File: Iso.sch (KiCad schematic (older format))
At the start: 16 parts, among them U11 SN74LVC2G14DBV, U12 4N35S, U13 4N35S, U14 SN74LVC2G14DBV

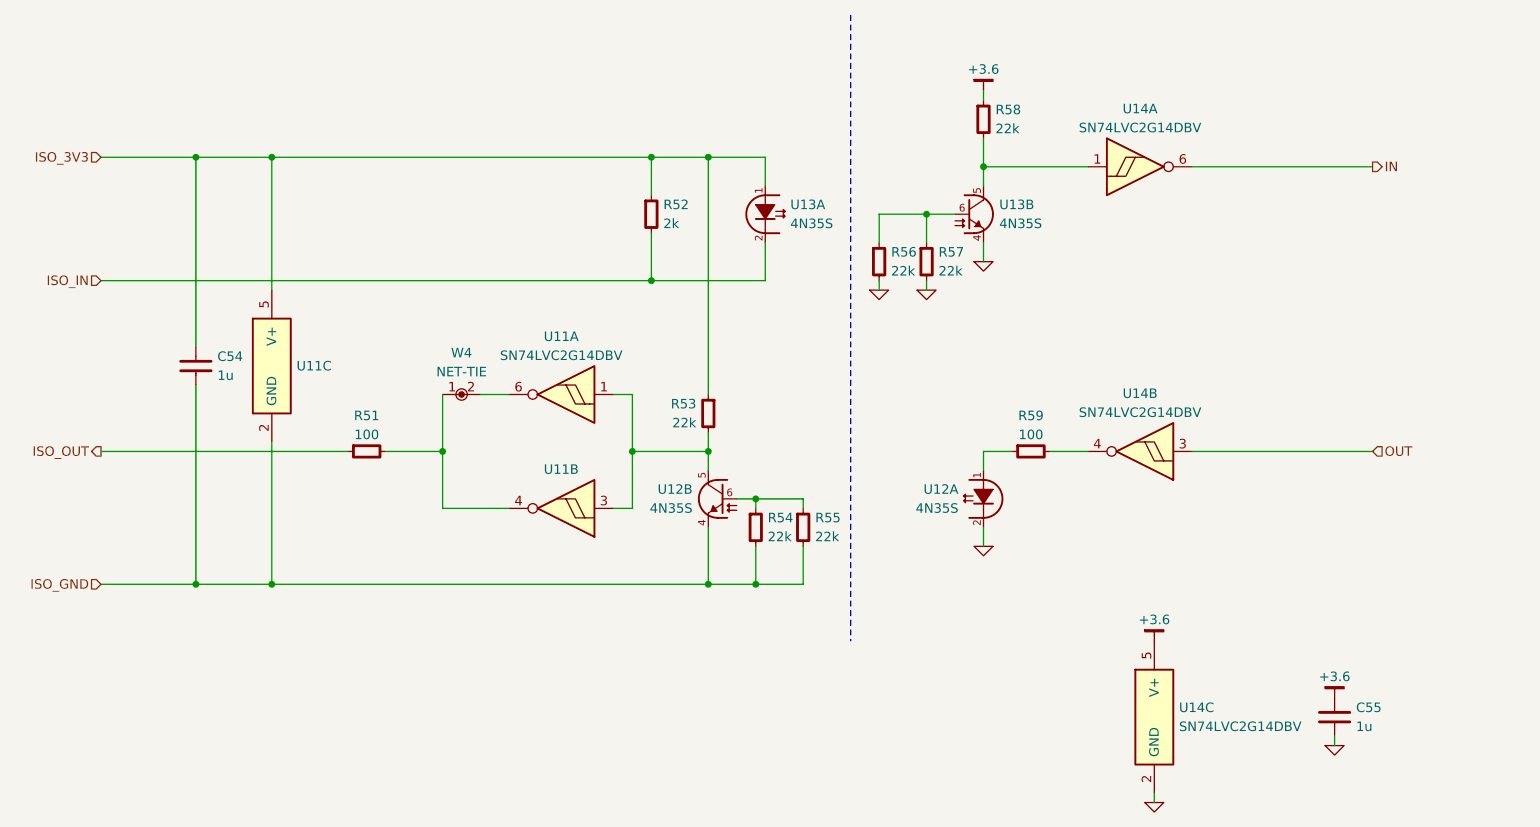
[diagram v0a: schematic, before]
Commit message: Piles and piles of work
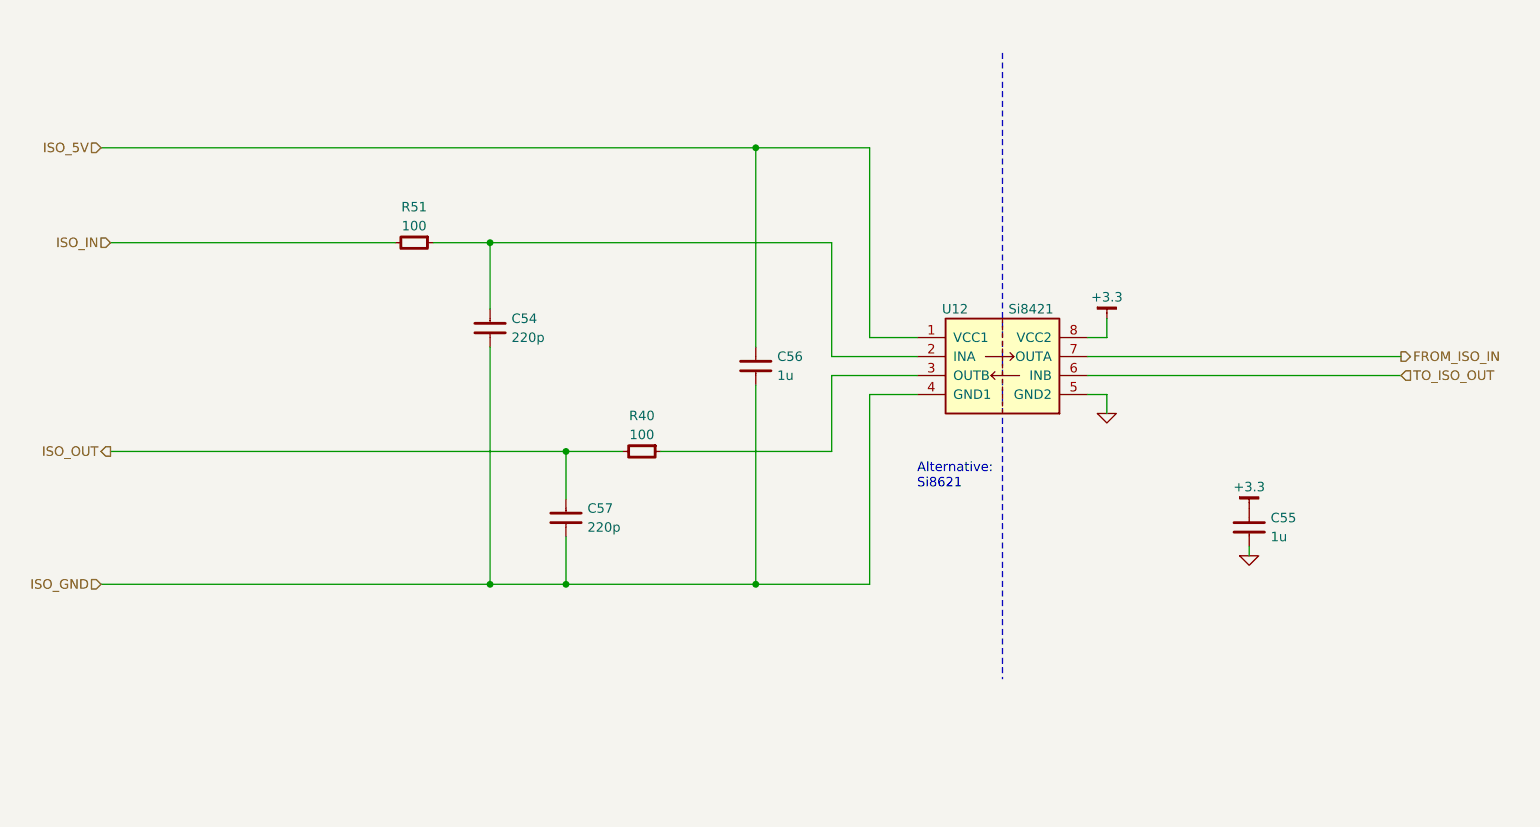
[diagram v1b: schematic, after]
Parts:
- removed C54: 1u, IPC7351-Nominal:CAPC2012X70, symbol C-0805
- removed R52: 2k, IPC7351-Nominal:RESC1608X50, symbol R-0603
- removed R53, R54, R55, R56, R57, R58: 22k, IPC7351-Nominal:RESC1608X50, symbol R-0603
- removed R59: 100, IPC7351-Nominal:RESC1608X50, symbol R-0603
- removed U11, U14: SN74LVC2G14DBV, smd-semi:SOT-23-6, symbol SN74LVC2G14DBV
- removed U12, U13: 4N35S, smd-semi:SOIC254P1016X460-6, symbol 4N35S
- removed W4: NET-TIE, conn-test:NET-TIE-0.3mm, symbol NET-TIE
- added C54, C57: 220p, IPC7351-Nominal:CAPC1608X55, symbol C-0603
- added C56: 1u, IPC7351-Nominal:CAPC2012X70, symbol C-0805
- added R40: 100, IPC7351-Nominal:RESC1608X50, symbol R-0603
- added U12: Si8421, IPC7351-Nominal:SOIC127P600X175-8, symbol Si8421
- R51: BOM RES SMD 100 5% [0603] -> RES SMD 100 1% [0603]
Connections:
- net GND: now also U12.5 (GND2)
- net ISO_GND: now also C54.1, C56.2, C57.1, U12.4 (GND1)
- net ISO_IN: now also R51.2
- net ISO_OUT: now also C57.2, R40.2; no longer R51.1
- net +3.6 renamed +3.3
- net +3.3: now also U12.8 (VCC2)
- new net: C54.2, R51.1, U12.2 (INA)
- new net: R40.1, U12.3 (OUTB)
- new net FROM_ISO_IN: U12.7 (OUTA)
- new net ISO_5V: C56.1, U12.1 (VCC1)
- new net TO_ISO_OUT: U12.6 (INB)
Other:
- note added: "Alternative:\nSi8621"
- moved on the sheet: C55
